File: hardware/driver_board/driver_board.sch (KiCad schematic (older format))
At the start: 99 parts, among them J1 796949-2, J2 796949-2, J3 796949-2, J4 796949-2, J5 Adafruit_1979, Q1 Toshiba_TK4R3E06PL, Q2 Toshiba_TK4R3E06PL, Q3 Toshiba_TK4R3E06PL, Q4 Toshiba_TK4R3E06PL, Q5 Toshiba_TK4R3E06PL, Q6 Toshiba_TK4R3E06PL, Q7 Toshiba_TK4R3E06PL, Q8 Toshiba_TK4R3E06PL, U1 HCPL-2631, U2 HCPL-2631, U3 IR2110, U4 IR2110, U5 IR2110, U6 IR2110, U7 LM7812_TO220, U8 MP1584EN

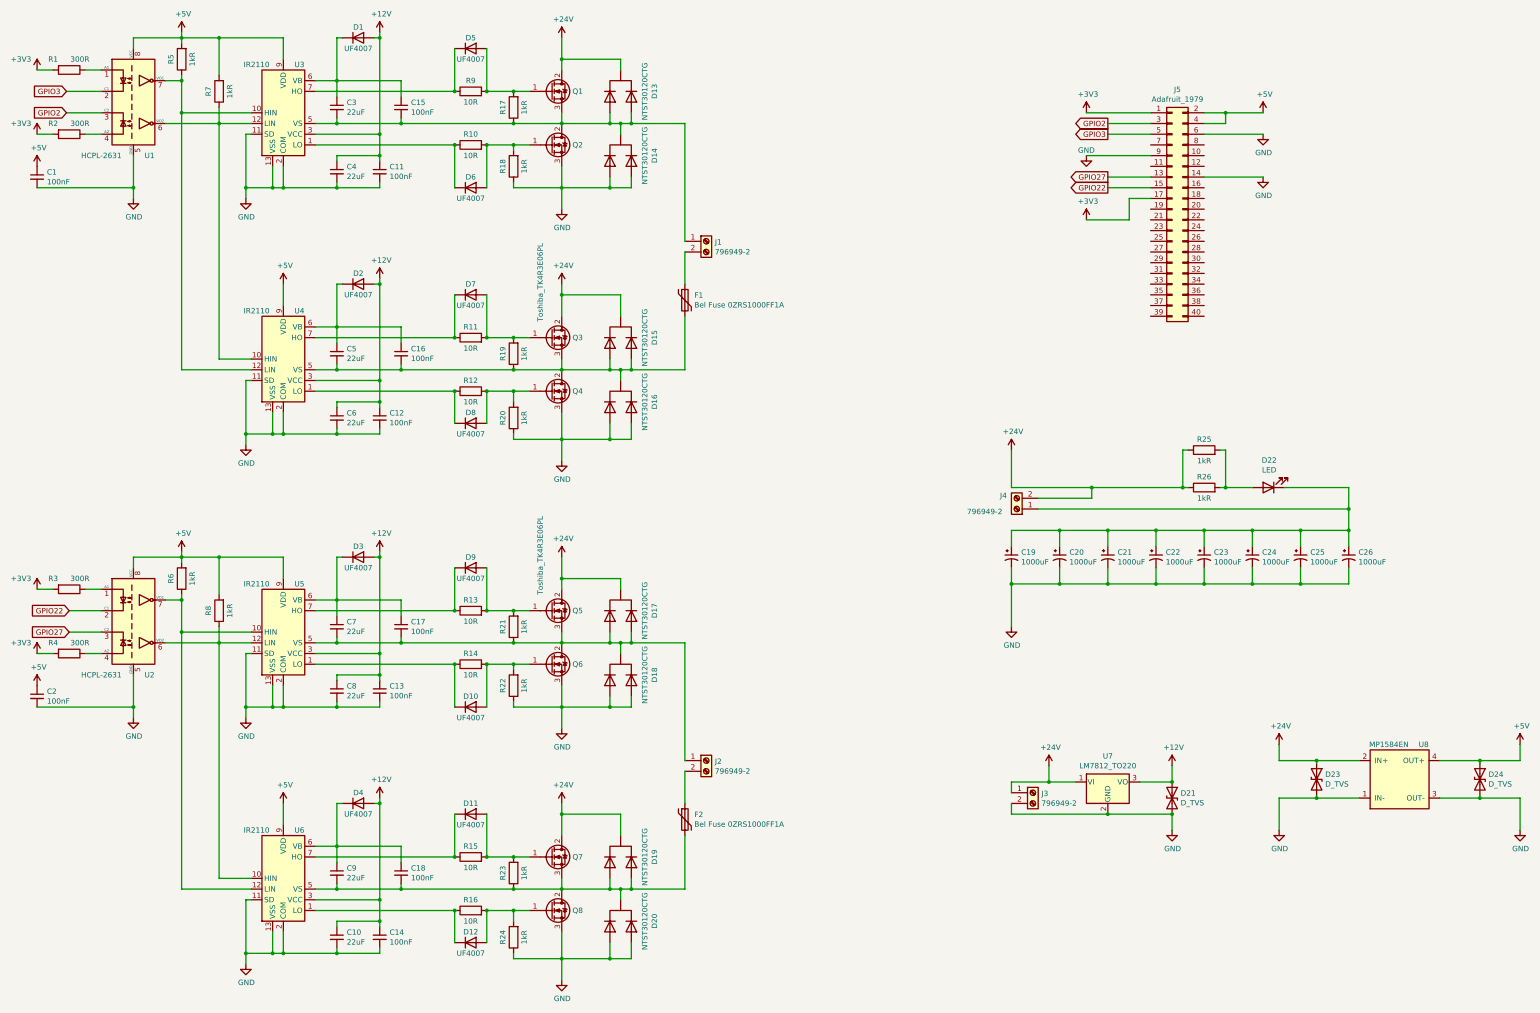
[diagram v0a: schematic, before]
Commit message: final update
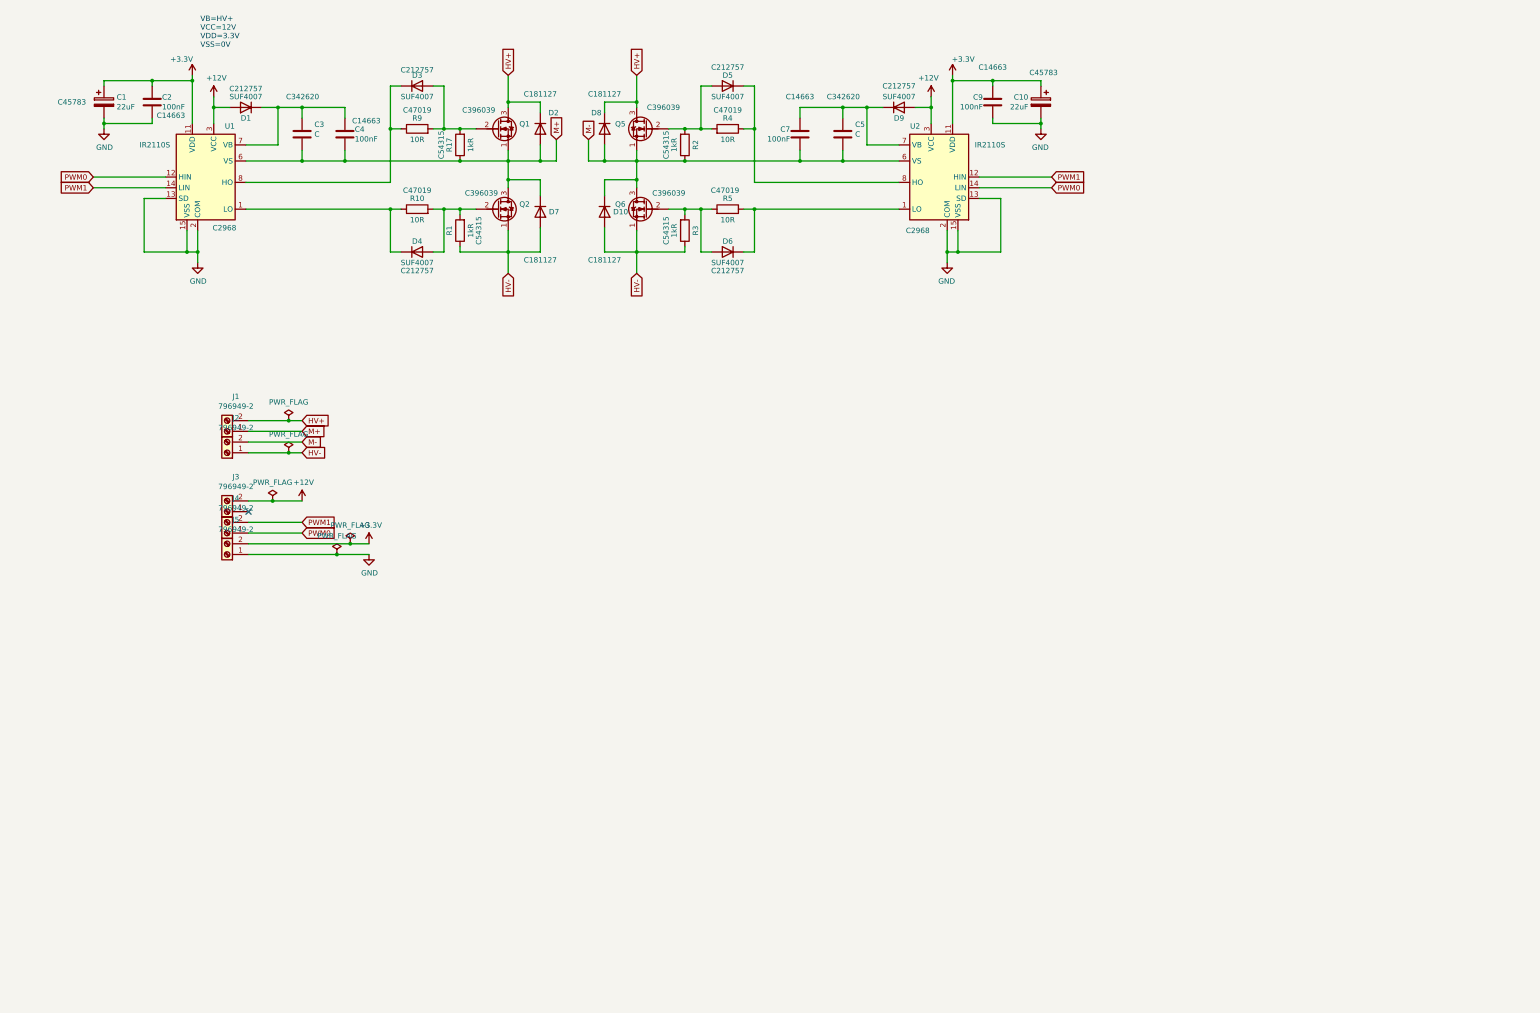
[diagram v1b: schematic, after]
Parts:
- removed C1, C11, C12, C13, C14, C15, C16, C17, C18, C2: 100nF, driver_board:C_Disc_D5.0mm_W2.5mm_P5.00mm, symbol Device:C_Small
- removed C10, C4, C6, C8: 22uF, driver_board:C_Disc_D5.1mm_W3.2mm_P5.00mm, symbol Device:C_Small
- removed C19, C20, C21, C22, C23, C24, C25, C26: 1000uF, driver_board:CP_Radial_D10.0mm_P5.00mm, symbol Device:CP1_Small
- removed C3, C5, C7, C9: 22uF, driver_board:C_Rect_L29.0mm_W11.0mm_P27.50mm_MKT, symbol Device:C_Small
- removed D11, D12: UF4007, Diode_THT:D_DO-41_SOD81_P10.16mm_Horizontal, symbol Diode:1N4007
- removed D13, D14, D15, D16, D17, D18, D19, D20: NTST30120CTG, driver_board:NTST30120CTG, symbol driver_board:NTST30120CTG
- removed D21, D23, D24: D_TVS, driver_board:D_DO-15_P10.16mm_Horizontal, symbol Device:D_TVS
- removed D22: LED, driver_board:LED_D5.0mm_PRECAHRGE, symbol Device:LED
- removed F1, F2: Bel Fuse 0ZRS1000FF1A, driver_board:RV_Disc_D21.5mm_W4.3mm_P10mm, symbol Device:Polyfuse
- removed J5: Adafruit_1979, driver_board:Adafruit_1979, symbol driver_board:Adafruit_1979
- removed Q1, Q2, Q3, Q4, Q5, Q6, Q7, Q8: Toshiba_TK4R3E06PL, driver_board:TK4R3E06RL, symbol driver_board:Toshiba_TK4R3E06PL
- removed R11, R12, R13, R14, R15, R16: 10R, driver_board:R_Axial_DIN0207_L6.3mm_D2.5mm_P7.62mm_Horizontal, symbol Device:R
- removed R18, R19, R20, R21, R22, R23, R24, R6, R7, R8: 1kR, driver_board:R_Axial_DIN0414_L11.9mm_D4.5mm_P15.24mm_Horizontal, symbol Device:R
- removed R25, R26: 1kR, driver_board:R_Axial_Power_L50.0mm_W9.0mm_P55.88mm, symbol Device:R
- removed U1, U2: HCPL-2631, Package_DIP:DIP-8_W7.62mm, symbol Isolator:HCPL-2631
- removed U3, U4, U5, U6: IR2110, Package_DIP:DIP-14_W7.62mm, symbol Driver_FET:IR2110
- removed U7: LM7812_TO220, Package_TO_SOT_THT:TO-220-3_Vertical, symbol Regulator_Linear:LM7812_TO220
- removed U8: MP1584EN, driver_board:MP1584, symbol driver_board:MP1584EN
- added C1, C10: 22uF, Capacitor_SMD:C_0805_2012Metric, symbol Device:CP
- added C2, C4, C7, C9: 100nF, Capacitor_SMD:C_0603_1608Metric, symbol Device:C
- added C3, C5: C, Capacitor_SMD:C_1206_3216Metric, symbol Device:C
- added J5: 796949-2, TerminalBlock_Phoenix:TerminalBlock_Phoenix_MKDS-1,5-2-5.08_1x02_P5.08mm_Horizontal, symbol driver_board:796949-2
- added Q1, Q2, Q5, Q6: TPH4R008NH,L1Q(M, driver_board:TPH4R008NH,L1Q(M, symbol driver_board:TPH4R008NH,L1Q(M
- added U1, U2: IR2110S, Package_SO:SOIC-16W_7.5x10.3mm_P1.27mm, symbol driver_board:IR2110S
- D1, D3, D4, D5, D6, D9: value UF4007 -> SUF4007; footprint Diode_THT:D_DO-41_SOD81_P10.16mm_Horizontal -> Diode_SMD:D_MELF; LCSC (none) -> C212757
- D10, D2, D7, D8: value UF4007 -> 1N4007; footprint Diode_THT:D_DO-41_SOD81_P10.16mm_Horizontal -> Diode_SMD:D_SOD-123F; LCSC (none) -> C181127
- J1, J2, J3, J4: footprint driver_board:796949-2 -> TerminalBlock_Phoenix:TerminalBlock_Phoenix_MKDS-1,5-2-5.08_1x02_P5.08mm_Horizontal
- R1, R2, R3: value 300R -> 1kR; footprint driver_board:R_Axial_DIN0207_L6.3mm_D2.5mm_P7.62mm_Horizontal -> Resistor_SMD:R_2512_6332Metric; LCSC (none) -> C54315
- R10, R9: footprint driver_board:R_Axial_DIN0207_L6.3mm_D2.5mm_P7.62mm_Horizontal -> Resistor_SMD:R_2512_6332Metric; LCSC (none) -> C47019
- R17: footprint driver_board:R_Axial_DIN0414_L11.9mm_D4.5mm_P15.24mm_Horizontal -> Resistor_SMD:R_2512_6332Metric; LCSC (none) -> C54315
- R4: value 300R -> 10R; footprint driver_board:R_Axial_DIN0207_L6.3mm_D2.5mm_P7.62mm_Horizontal -> Resistor_SMD:R_2512_6332Metric; LCSC (none) -> C47019
- R5: value 1kR -> 10R; footprint driver_board:R_Axial_DIN0414_L11.9mm_D4.5mm_P15.24mm_Horizontal -> Resistor_SMD:R_2512_6332Metric; LCSC (none) -> C47019
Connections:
- net +12V: now also D9.2 (A), J3.2 (Pin_2), U1.3 (VCC), U2.3 (VCC); no longer D2.2 (A), D3.2 (A), D4.2 (A)
- net +3V3: now also C1.1, C10.1, C2.1, C9.1, J5.2 (Pin_2), U1.11 (VDD), U2.11 (VDD); no longer R1.2, R2.2, R3.2, R4.2
- net GND: now also C1.2, C10.2, C2.2, C9.2, J5.1 (Pin_1), U1.13 (SD), U1.15 (VSS), U1.2 (COM), U2.13 (SD), U2.15 (VSS), U2.2 (COM); no longer J3.2 (Pin_2)
- net HV+: now reaches D8.1 (K)
- net HV+: now also D2.1 (K), J1.2 (Pin_2), Q1.3 (D), Q5.3 (D)
- net at R5.1: now also D6.1 (K), U2.1 (LO)
- net M+: now reaches D7.1 (K)
- net M+: now also D2.2 (A), J1.1 (Pin_1), R17.1, C3.2, C4.2, Q1.1 (S), Q2.3 (D), U1.6 (VS)
- net M-: now reaches D8.2 (A)
- net M-: now also D10.1 (K), J2.2 (Pin_2), R2.1, C5.2, C7.2, Q5.1 (S), Q6.3 (D), U2.6 (VS)
- net HV-: now reaches D7.2 (A)
- net HV-: now also D10.2 (A), J2.1 (Pin_1), R1.1, R3.1, Q2.1 (S), Q6.1 (S)
- net at R10.1: now also D4.1 (K), U1.1 (LO); no longer D6.1 (K)
- net at D1.1 (K): now also C3.1, C4.1, U1.7 (VB)
- net at R9.1: now also D3.1 (K), U1.8 (HO); no longer D5.1 (K)
- net at R10.2: now also D4.2 (A), R1.2, Q2.2 (G); no longer D6.2 (A)
- net at R17.2, R9.2: now also D3.2 (A), Q1.2 (G); no longer D5.2 (A)
- net at R4.1: now also D5.1 (K), U2.8 (HO)
- net PWM0: now reaches J4.1 (Pin_1)
- net PWM0: now also U1.12 (HIN), U2.14 (LIN)
- net at D9.1 (K): now also C5.1, C7.1, U2.7 (VB)
- net +24V: no longer names the net of J3.1 (Pin_1)
- net +24V: no longer J4.2 (Pin_2)
- net +5V: no longer names the net of R5.2
- net +5V: now also D6.2 (A), R3.2, Q6.2 (G)
- new net: D5.2 (A), Q5.2 (G), R2.2, R4.2
- new net PWM1: J4.2 (Pin_2), U1.14 (LIN), U2.12 (HIN)
- no-connect marks 0 -> 1
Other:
- note added: "VB=HV+\nVCC=12V\nVDD=3.3V\nVSS=0V\n"
- moved on the sheet: D1, R10, R17, R9

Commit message: update
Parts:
- Q1, Q2, Q5, Q6: footprint driver_board:TPH4R008NH,L1Q(M -> driver_board:SOP-8-1EP_4.57x4.57mm_P1.27mm_EP4.57x4.45mm_ThermalVias
- U1, U2: footprint Package_SO:SOIC-16W_7.5x10.3mm_P1.27mm -> driver_board:SOIC-16W_7.5x10.3mm_P1.27mm_R90
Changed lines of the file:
@@
 F 0 "U1" H 2950 3325 50  0000 C CNN
 F 1 "IR2110S" H 2250 3150 50  0000 C CNN
-F 2 "Package_SO:SOIC-16W_7.5x10.3mm_P1.27mm" H 2800 2850 50  0001 C CIN
+F 2 "driver_board:SOIC-16W_7.5x10.3mm_P1.27mm_R90" H 2800 2850 50  0001 C CIN
 F 3 "https://www.infineon.com/dgdl/ir2110.pdf?fileId=5546d462533600a4015355c80333167e" H 2650 2850 50  0001 C CNN
 F 4 "C2968" H 2900 2375 50  0000 C CNN "LCSC"
@@
 F 0 "Q1" H 5654 2446 50  0000 L CNN
 F 1 "TPH4R008NH,L1Q(M" V 5325 2575 50  0001 L CNN
-F 2 "driver_board:TPH4R008NH,L1Q(M" H 5650 2500 50  0001 C CNN
+F 2 "driver_board:SOP-8-1EP_4.57x4.57mm_P1.27mm_EP4.57x4.45mm_ThermalVias" H 5650 2500 50  0001 C CNN
 F 3 "https://www.mouser.com/datasheet/2/408/TPH4R008NH_datasheet_en_20191017-1140027.pdf" H 5450 2400 50  0001 C CNN
 F 4 "C396039" H 5275 2575 50  0000 C CNN "LCSC"
@@
 F 0 "Q2" H 5654 3196 50  0000 L CNN
 F 1 "TPH4R008NH,L1Q(M" V 5325 3325 50  0001 L CNN
-F 2 "driver_board:TPH4R008NH,L1Q(M" H 5650 3250 50  0001 C CNN
+F 2 "driver_board:SOP-8-1EP_4.57x4.57mm_P1.27mm_EP4.57x4.45mm_ThermalVias" H 5650 3250 50  0001 C CNN
 F 3 "https://www.mouser.com/datasheet/2/408/TPH4R008NH_datasheet_en_20191017-1140027.pdf" H 5450 3150 50  0001 C CNN
 F 4 "C396039" H 5300 3300 50  0000 C CNN "LCSC"
@@
 F 0 "U2" H 9950 3325 50  0000 C CNN
 F 1 "IR2110S" H 9250 3150 50  0000 C CNN
-F 2 "Package_SO:SOIC-16W_7.5x10.3mm_P1.27mm" H 9800 2850 50  0001 C CIN
+F 2 "driver_board:SOIC-16W_7.5x10.3mm_P1.27mm_R90" H 9800 2850 50  0001 C CIN
 F 3 "https://www.infineon.com/dgdl/ir2110.pdf?fileId=5546d462533600a4015355c80333167e" H 9650 2850 50  0001 C CNN
 F 4 "C2968" H 9925 2350 50  0000 C CNN "LCSC"
@@
 F 0 "Q5" H 7054 2446 50  0000 L CNN
 F 1 "TPH4R008NH,L1Q(M" V 6725 2575 50  0001 L CNN
-F 2 "driver_board:TPH4R008NH,L1Q(M" H 7050 2500 50  0001 C CNN
+F 2 "driver_board:SOP-8-1EP_4.57x4.57mm_P1.27mm_EP4.57x4.45mm_ThermalVias" H 7050 2500 50  0001 C CNN
 F 3 "https://www.mouser.com/datasheet/2/408/TPH4R008NH_datasheet_en_20191017-1140027.pdf" H 6850 2400 50  0001 C CNN
 F 4 "C396039" H 6700 2600 50  0000 C CNN "LCSC"
@@
 F 0 "Q6" H 7054 3196 50  0000 L CNN
 F 1 "TPH4R008NH,L1Q(M" V 6725 3325 50  0001 L CNN
-F 2 "driver_board:TPH4R008NH,L1Q(M" H 7050 3250 50  0001 C CNN
+F 2 "driver_board:SOP-8-1EP_4.57x4.57mm_P1.27mm_EP4.57x4.45mm_ThermalVias" H 7050 3250 50  0001 C CNN
 F 3 "https://www.mouser.com/datasheet/2/408/TPH4R008NH_datasheet_en_20191017-1140027.pdf" H 6850 3150 50  0001 C CNN
 F 4 "C396039" H 6650 3300 50  0000 C CNN "LCSC"
